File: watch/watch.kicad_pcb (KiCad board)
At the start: 2 copper layers, 40 x 40 mm, 95 parts, among them IC1 IS32FL3237-TQLA3-TR, IC2 TMUX1237DCKR, SW1 ButtonWakeup, SW2 ButtonUp, SW3 ButtonDown, U1 STM32L031F4Px, Y1 CR_32kHz

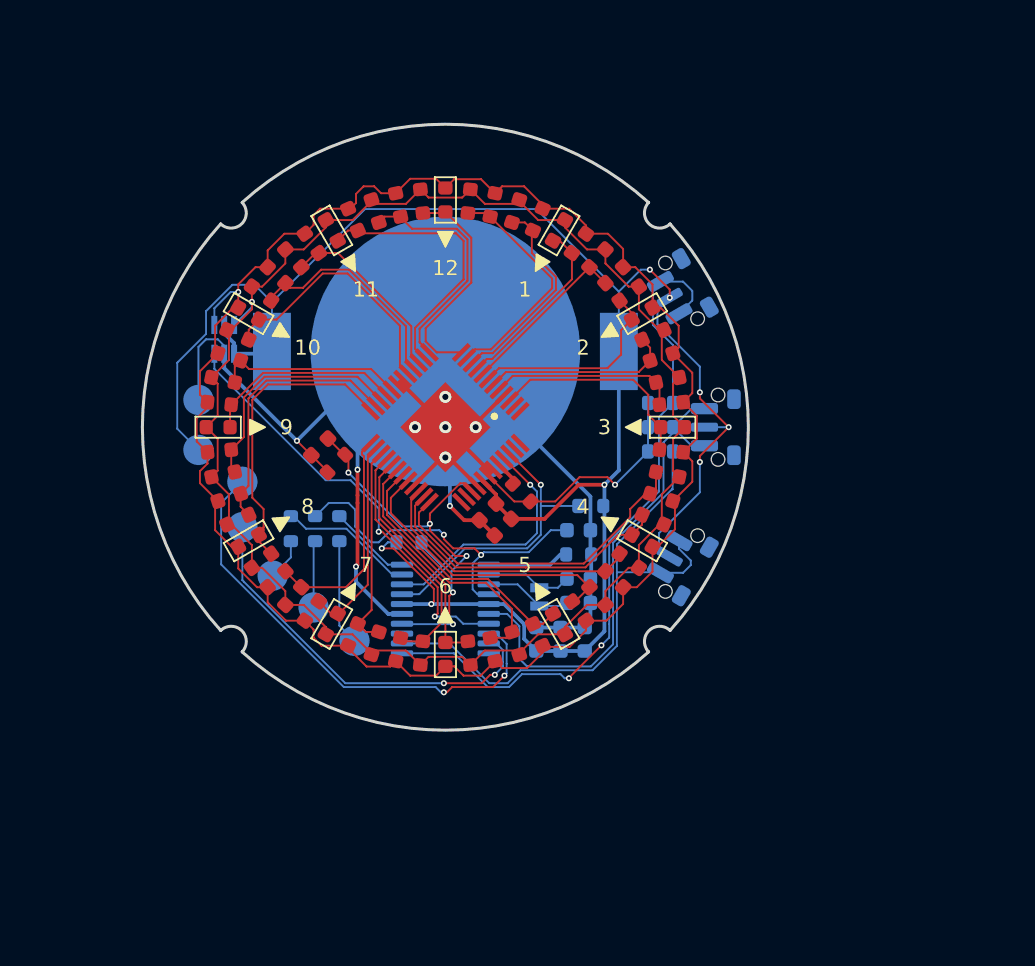
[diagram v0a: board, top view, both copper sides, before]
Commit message: as ordered V1.4
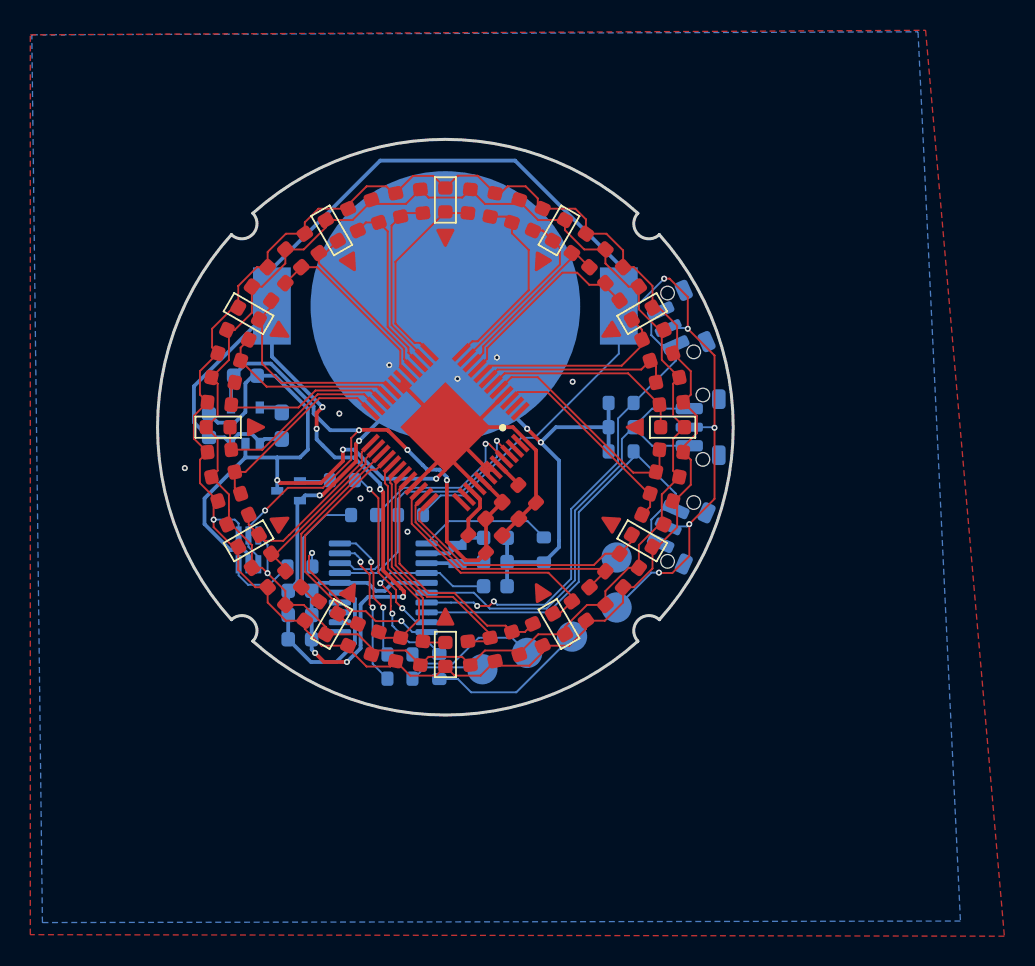
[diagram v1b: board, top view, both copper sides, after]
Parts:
- removed R28, R31: 2k, custom:R_0603_1608Metric
- removed TP6: UART_TX, TestPoint:TestPoint_Pad_D2.0mm
- removed TP7: UART_RX, TestPoint:TestPoint_Pad_D2.0mm
- added C10: 10uF, custom:C_0603_1608Metric, B.Cu at (86.8, 96.6)
- added L1: 4.7uH, Inductor_SMD:L_0603_1608Metric_Pad1.05x0.95mm_HandSolder, B.Cu at (89.2, 99.9)
- added Q1: RU1C002UNTCL, mrab:SOT-323FL, B.Cu at (89.7, 104.2)
- added R5: 2k, custom:R_0603_1608Metric, B.Cu at (97.7, 105.8)
- added R6: 2k, custom:R_0603_1608Metric, B.Cu at (94.6, 105.8)
- added R7: 10k, custom:R_0603_1608Metric, B.Cu at (90.4, 109.2)
- added R8: 2k, custom:R_0603_1608Metric, B.Cu at (93.2, 103.5)
- added VR1: XC9140331MR-G, mrab:SOT-25, B.Cu at (86.8, 99.9)
- BT1: footprint BAT-HLD-001:BATHLD001 -> SamacSys_Parts:BATHLD001
- C2: value 100nF -> 4.7uF; moved to B.Cu
- TP1: value SWD_3V3 -> SWD_BAT
- moved TP1 29.5 mm to (111.3, 111.9)
- moved TP2 29.5 mm to (111.3, 108.6)
- moved C5 18.8 mm to (90.4, 114.0), turned to 0 degrees
- moved C7 17.5 mm to (90.4, 110.8), turned to 0 degrees
- moved TP5 17.2 mm to (108.4, 113.8), turned to 20 degrees
- moved C6 15.7 mm to (90.4, 112.4), turned to 0 degrees
- moved TP3 15.2 mm to (102.4, 116.0), turned to 20 degrees
- moved IC2 14.0 mm to (87.0, 108.1)
- moved R3 12.2 mm to (99.6, 115.8)
- moved R1 12.2 mm to (97.0, 116.6), turned to 0 degrees
- moved TP4 11.4 mm to (105.4, 114.9), turned to 20 degrees
- moved R20 10.7 mm to (102.1, 107.7), turned to -45 degrees
- moved R2 9.21 mm to (97.0, 115.0), turned to 0 degrees
- moved C2 7.43 mm to (84.4, 99.9), turned to 90 degrees
- moved C1 6.63 mm to (103.3, 110.5)
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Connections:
- BT1 pad 1: +3V3 -> +BATT
- C2 pad 1: /LED_Driver/EN -> +BATT
- C2 pad 2: GND -> GND1
- C3 pad 1: GND -> GND1
- C3 pad 2: +3V3 -> /LED_Driver/VCC_LED
- C4 pad 1: GND -> GND1
- C4 pad 2: +3V3 -> /LED_Driver/VCC_LED
- C5 pad 2: +3V3 -> +BATT
- C6 pad 2: +3V3 -> +BATT
- C7 pad 2: +3V3 -> +BATT
- IC1 pad 18: GND -> GND1
- IC1 pad 19: GND -> GND1
- IC1 pad 33: GND -> GND1
- IC1 pad 39: /LED_Driver/EN -> Net-(IC1-Pad39)
- IC1 pad 4: GND -> GND1
- IC1 pad 40: GND -> GND1
- IC1 pad 41: +3V3 -> /LED_Driver/VCC_LED
- IC1 pad 42: GND -> GND1
- IC1 pad 43: GND -> GND1
- IC1 pad 49: GND -> GND1
- IC2 pad 2: +3V3 -> /LED_Driver/VCC_LED
- IC2 pad 4: +3V3 -> /LED_Driver/VCC_LED
- IC2 pad 5: GND -> GND1
- IC2 pad 6: /LED_Driver/LED_BANK -> Net-(IC2-Pad6)
- R20 pad 1: /LED_Driver/EN -> Net-(IC1-Pad39)
- R20 pad 2: GND -> /LED_Driver/VCC_LED
- R24 pad 1: GND -> GND1
- SW1 pad 2: +3V3 -> +BATT
- SW2 pad 2: +3V3 -> +BATT
- SW3 pad 2: +3V3 -> +BATT
- TP1 pad 1: +3V3 -> +BATT
- U1 pad 10: unconnected-(U1-Pad10) -> /LED_Driver/LED_BANK
- U1 pad 11: Net-(R45-Pad1) -> unconnected-(U1-Pad11)
- U1 pad 12: Net-(R46-Pad1) -> unconnected-(U1-Pad12)
- U1 pad 14: /LED_Driver/EN -> unconnected-(U1-Pad14)
- U1 pad 16: +3V3 -> +BATT
- U1 pad 5: +3V3 -> +BATT
- U1 pad 7: /LED_Driver/LED_BANK -> Net-(R45-Pad1)
- U1 pad 8: Net-(TP6-Pad1) -> Net-(R46-Pad1)
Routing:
- net +BATT: track 0.00 -> 161.0 mm, vias 0 -> 11
- net +3V3: track 135.5 -> 0.00 mm, vias 8 -> 0
- net GND1: track 0.00 -> 81.6 mm, vias 0 -> 3
- net GND: track 129.5 -> 75.5 mm, vias 10 -> 12
- net /LED_Driver/VCC_LED: track 0.00 -> 46.9 mm, vias 0 -> 4
- net Net-(TP6-Pad1): track 32.3 -> 0.00 mm, vias 2 -> 0
- net /LED_Driver/EN: track 26.4 -> 0.00 mm, vias 5 -> 0
- net /LED_Driver/LED_BANK: track 28.4 -> 12.4 mm
- net Net-(R45-Pad1): track 47.2 -> 32.6 mm
- net Net-(U1-Pad9): track 26.2 -> 12.0 mm
- net nRST: track 24.3 -> 14.7 mm
- net Net-(R46-Pad1): track 37.7 -> 29.9 mm
- net Net-(D21-Pad1): track 20.6 -> 12.9 mm
- net Net-(R3-Pad2): track 4.42 -> 10.6 mm
- net Net-(D5-Pad1): track 18.2 -> 12.0 mm
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- added copper zone on B.Cu, net GND
- added copper zone on F.Cu, net GND
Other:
- board size 40 x 40 mm -> 38 x 38 mm
- board text added: "SWDCLK"
- board text added: "SWDIO"
- board text added: "SWDRST"
- board text added: "V1.4"
- board text removed: "1"
- board text removed: "10"
- board text removed: "11"
- board text removed: "12"
- board text removed: "2"
- board text removed: "3"
- board text removed: "4"
- board text removed: "5"
- board text removed: "6"
- board text removed: "7"
- board text removed: "8"
- board text removed: "9"
- board text removed: "RX"
- board text removed: "SWCLK"
- board text removed: "SWIO"
- board text removed: "SWRST"
- board text removed: "TX"
- board text removed: "V1.2"
